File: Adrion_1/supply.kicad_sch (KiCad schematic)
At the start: 25 parts, among them IC2 L6986H, IC3 TPS7A2030PDBVR, U7 TLV9001IDCKR

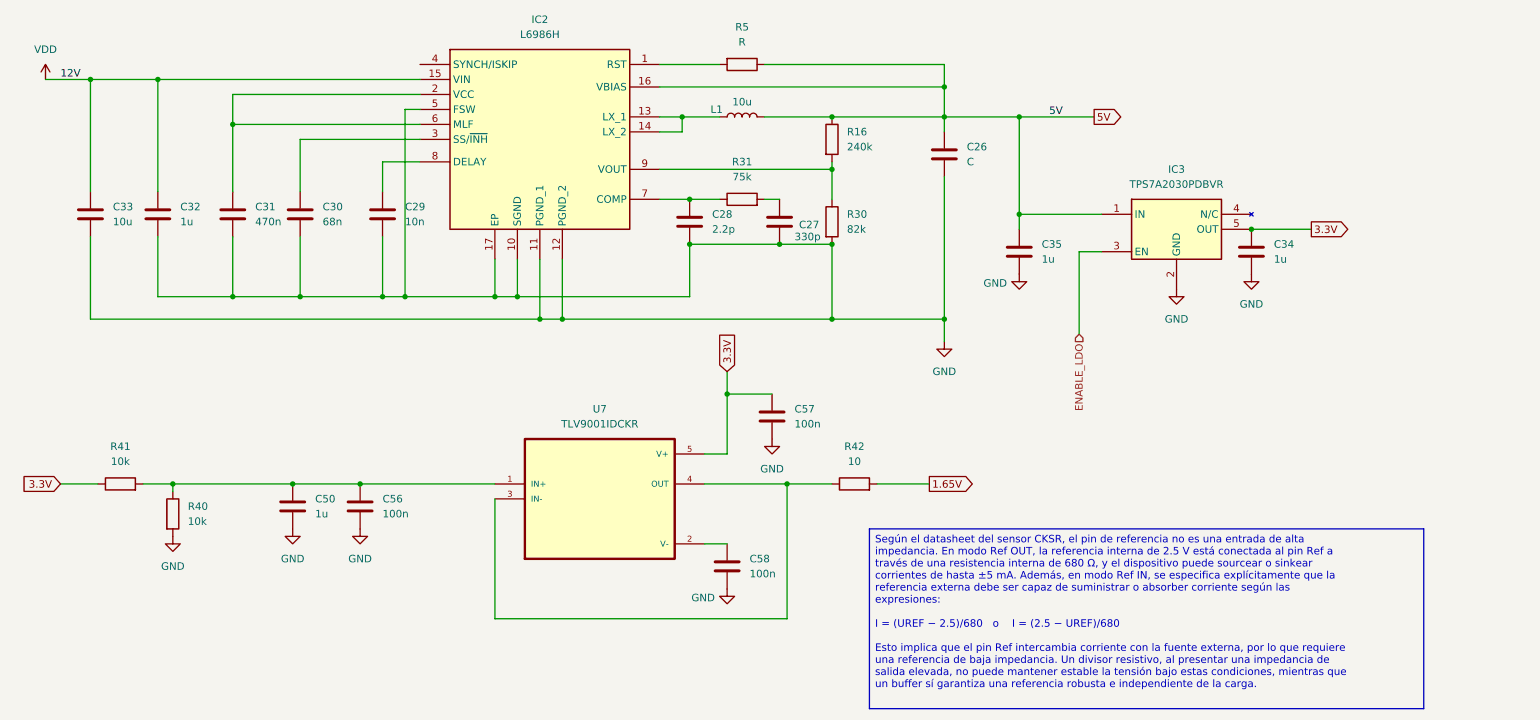
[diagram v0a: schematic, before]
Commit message: Correcion railes de tension papa
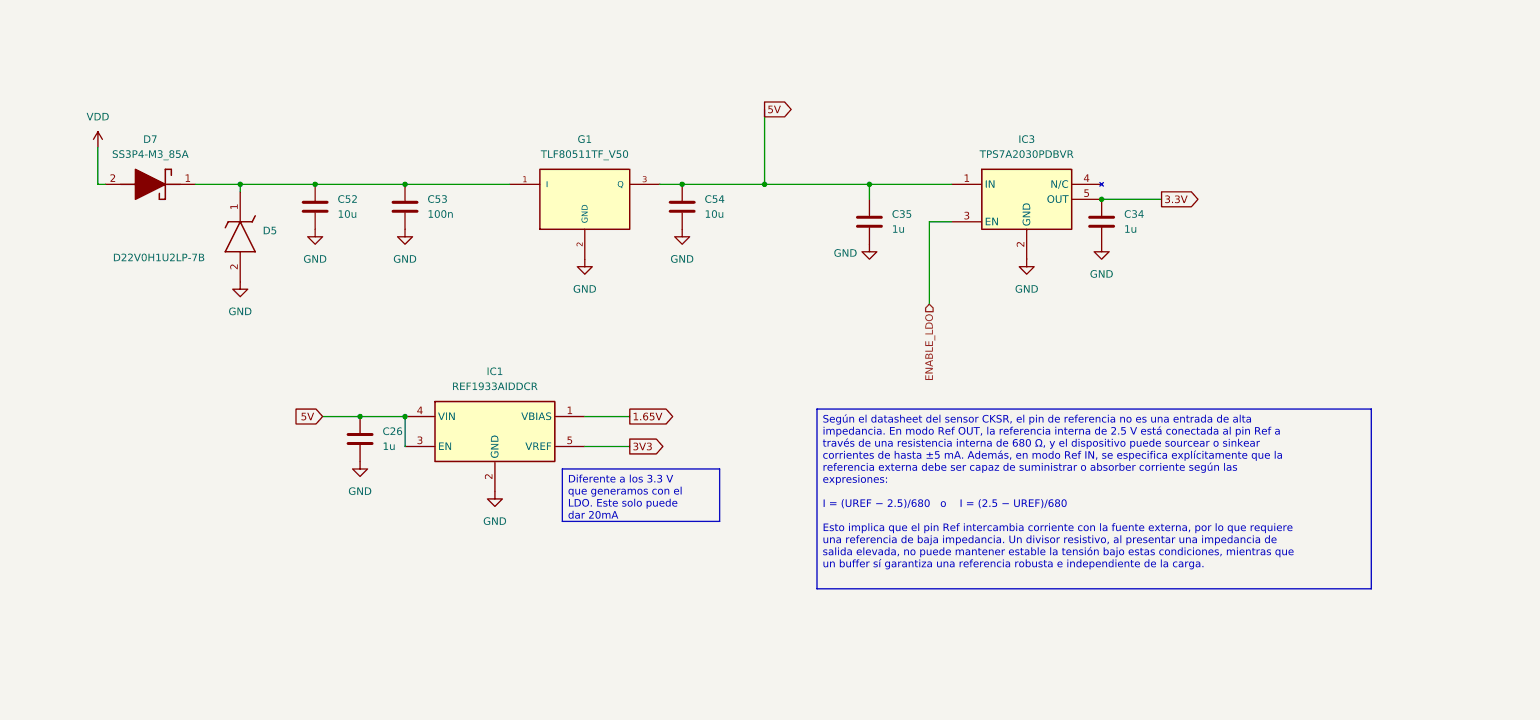
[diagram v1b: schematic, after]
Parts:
- removed C27: 330p, symbol Device:C
- removed C28: 2.2p, symbol Device:C
- removed C29: 10n, symbol Device:C
- removed C30: 68n, symbol Device:C
- removed C31: 470n, symbol Device:C
- removed C32, C50: 1u, symbol Device:C
- removed C33: 10u, symbol Device:C
- removed C56, C57, C58: 100n, symbol Device:C
- removed IC2: L6986H, SOP65P640X120-17N, symbol L6986H:L6986H
- removed L1: 10u, symbol Device:L
- removed R16: 240k, symbol Device:R
- removed R30: 82k, symbol Device:R
- removed R31: 75k, symbol Device:R
- removed R40, R41: 10k, symbol Device:R
- removed R42: 10, symbol Device:R
- removed R5: R, symbol Device:R
- removed U7: TLV9001IDCKR, TLV9001IDCKR:SOT65P210X110-5N, symbol TLV9001IDCKR:TLV9001IDCKR
- added C52, C54: 10u, symbol Device:C
- added C53: 100n, symbol Device:C
- added D5: D22V0H1U2LP-7B, D22V0H1U2LP7B, symbol D22V0H1U2LP-7B:D22V0H1U2LP-7B
- added D7: SS3P4-M3_85A, SS3P4M385A, symbol SS3P4-M3_85A:SS3P4-M3_85A
- added G1: TLF80511TF_V50, TLF80511TF_V50:INF-PG-TO252-3-11_N, symbol TLF80511TF_V50:TLF80511TF_V50
- added IC1: REF1933AIDDCR, SOT95P280X110-5N, symbol REF1933AIDDCR:REF1933AIDDCR
- C26: value C -> 1u
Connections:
- net 1.65V: now also IC1.1 (VBIAS)
- net 5V: now also C54.1, G1.3 (Q), IC1.3 (EN), IC1.4 (VIN)
- net GND: now also C52.2, C53.2, C54.2, D5.2 (A), G1.2 (GND), IC1.2 (GND)
- net VDD: now also D7.2 (A)
- new net: C52.1, C53.1, D5.1 (K), D7.1 (K), G1.1 (I)
- new net 3V3: IC1.5 (VREF)
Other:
- moved on the sheet: C34, C35, IC3
